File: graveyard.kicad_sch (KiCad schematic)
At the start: 93 parts, among them J30 TX_FILT_IN, J31 To CTRL:ATU, J32 UTF1_OUT, J33 UTF1_IN, J34 UTF1_OUT, J35 UTF1_IN, J36 TX_FILT_OUT, K35 EC2-5SNU, K36 EC2-5SNU, K37 EC2-5SNU, K38 EC2-5SNU, K39 EC2-5SNU, K40 EC2-5SNU, K41 EC2-5SNU, K42 EC2-5SNU, K43 G6E, K44 EC2-5SNU, Q10 BT169B, U17 ULN2803A, U18 MCP23008-xSO, U19 LM555xM

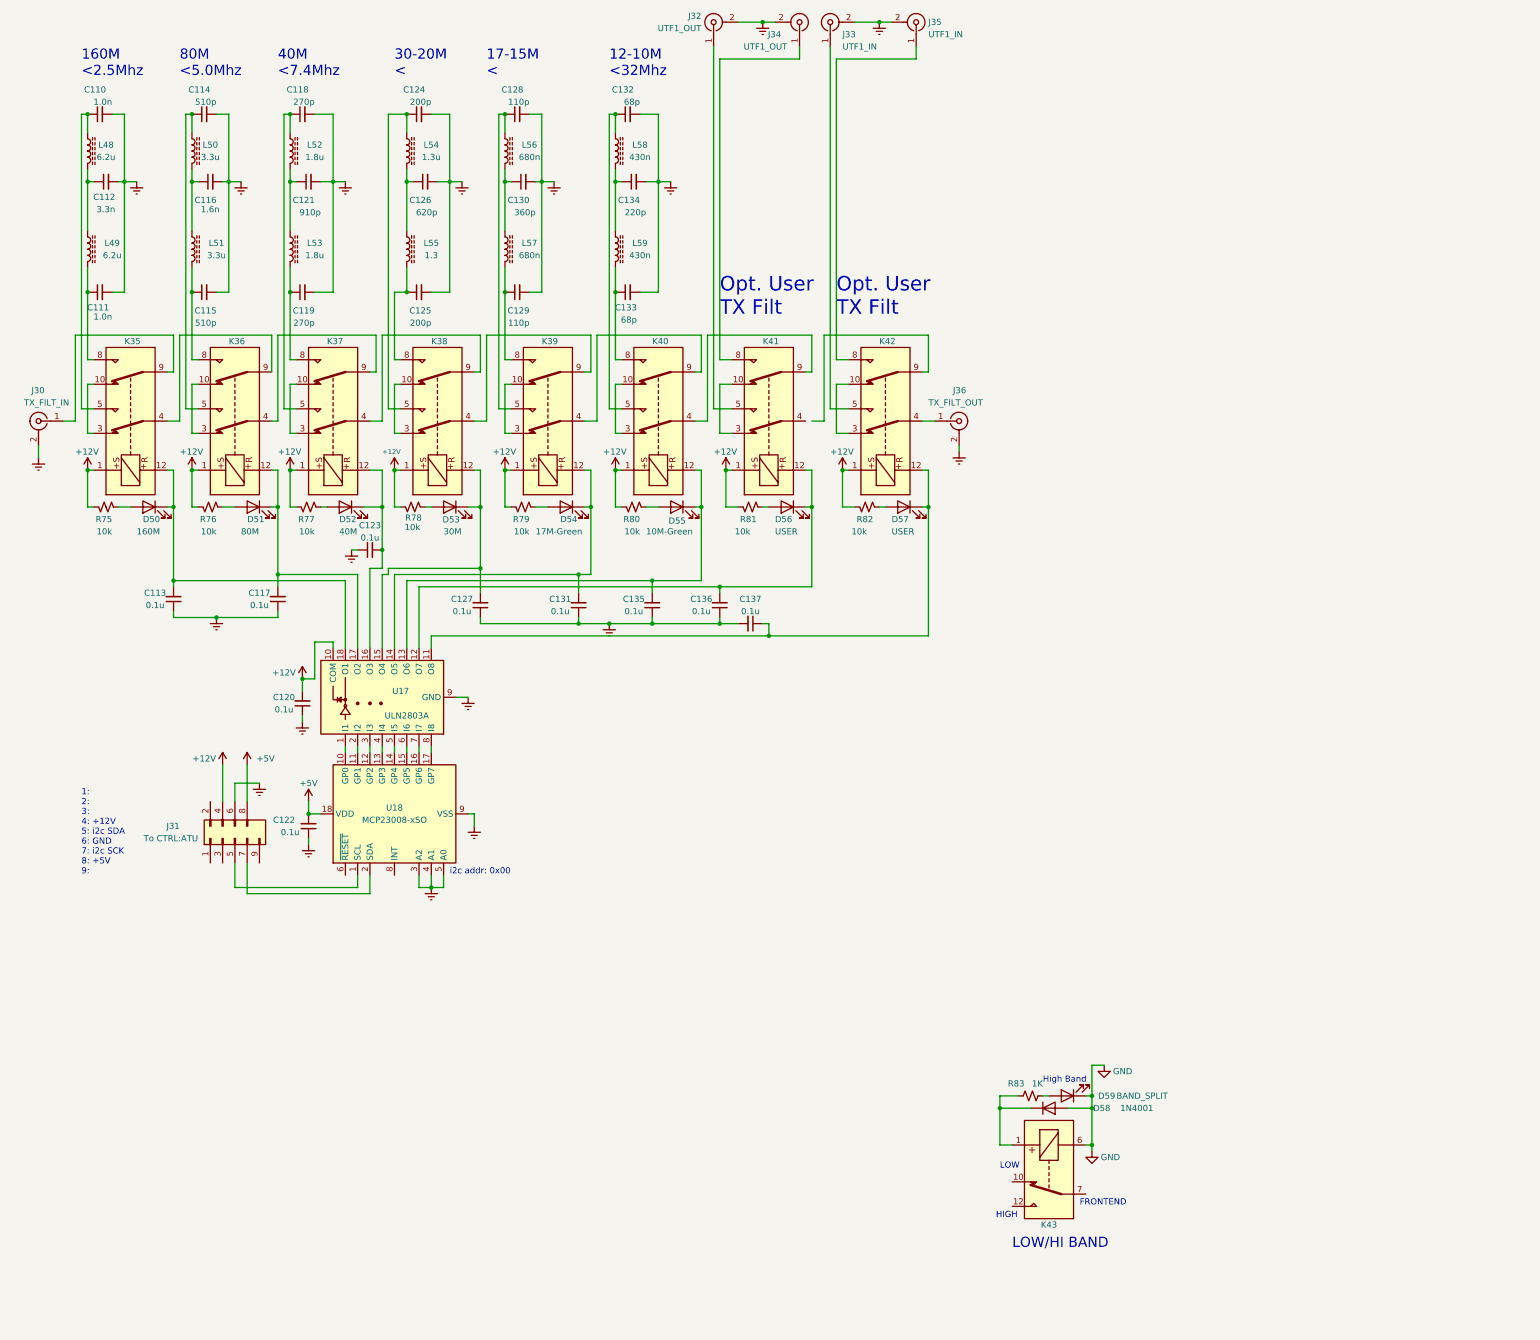
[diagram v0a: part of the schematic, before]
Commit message: cleanup of schematic and some initial firmware works...
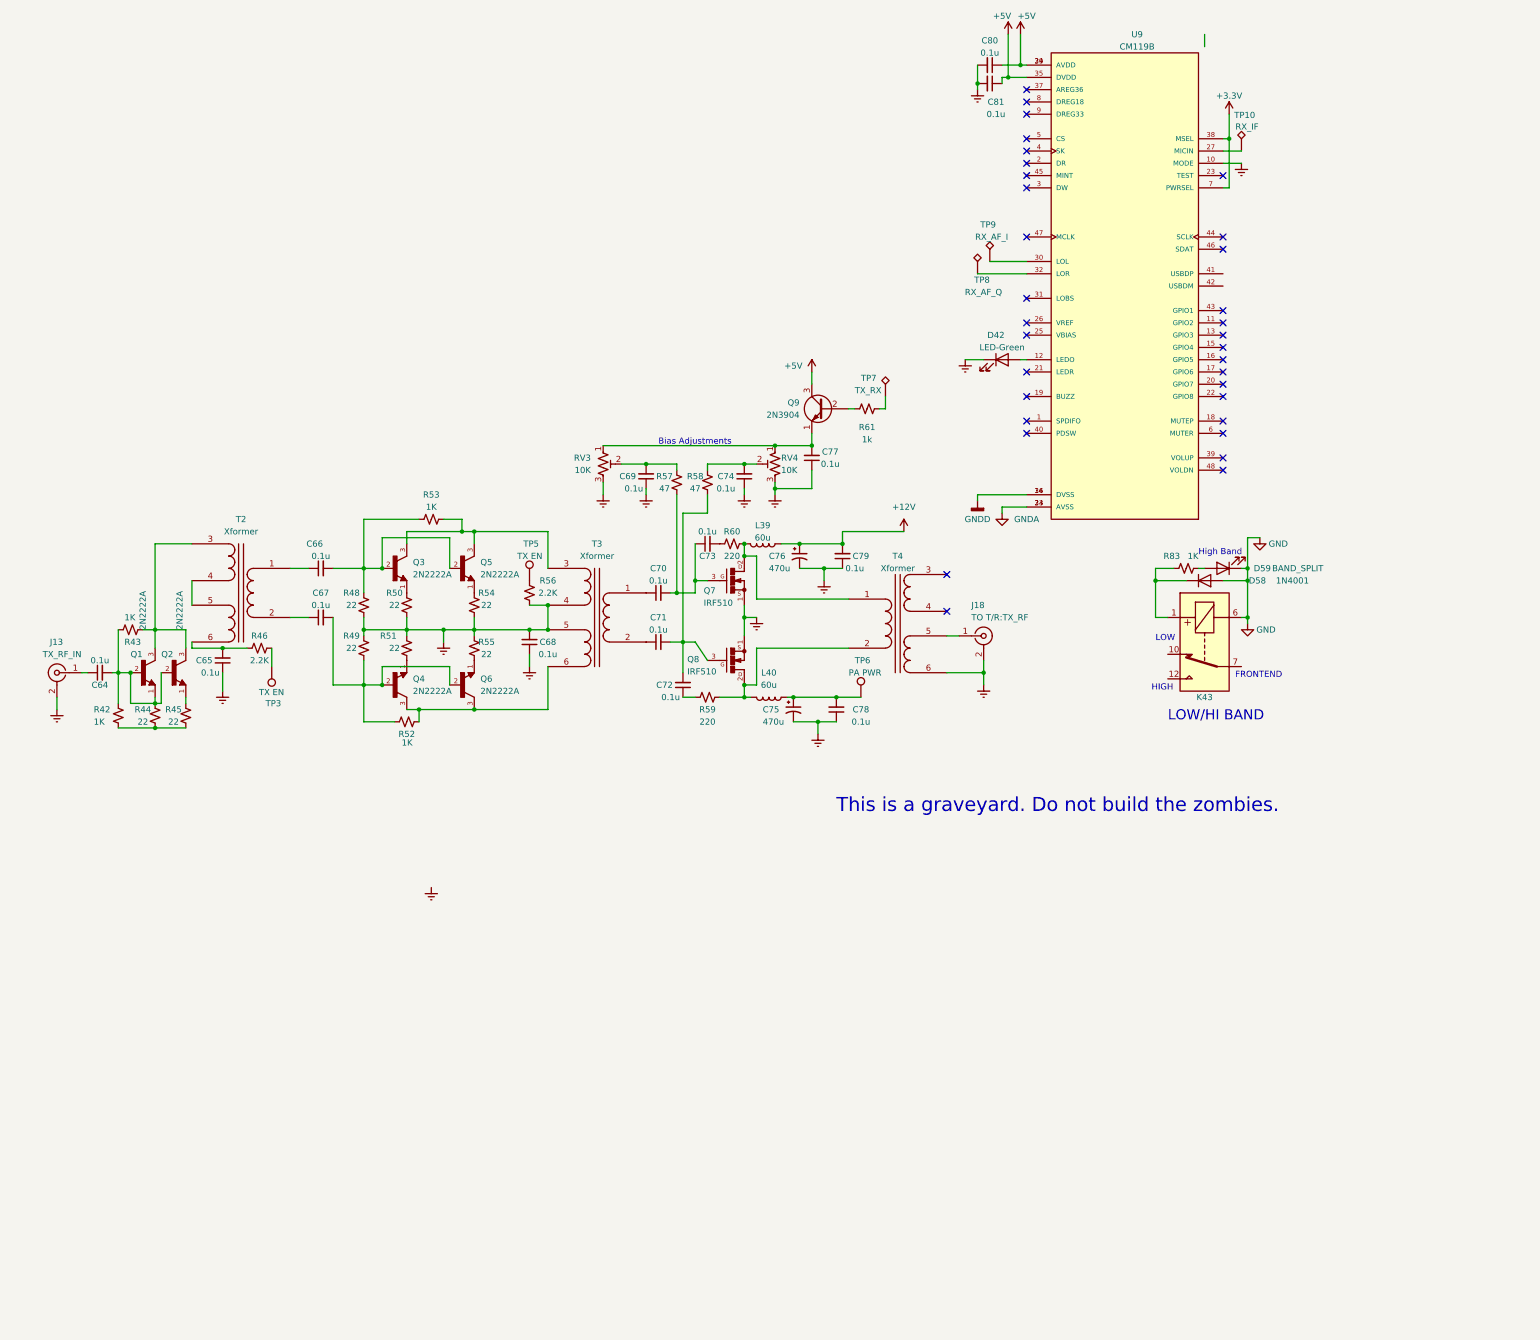
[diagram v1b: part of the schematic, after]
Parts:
- removed C110, C111: 1.0n, symbol Device:C_Small
- removed C112: 3.3n, symbol Device:C_Small
- removed C113, C117, C120, C122, C123, C127, C131, C135, C136, C137: 0.1u, Capacitor_THT:C_Disc_D4.7mm_W2.5mm_P5.00mm, symbol Device:C_Small
- removed C114, C115: 510p, symbol Device:C_Small
- removed C116: 1.6n, symbol Device:C_Small
- removed C118, C119: 270p, symbol Device:C_Small
- removed C121: 910p, symbol Device:C_Small
- removed C124, C125: 200p, symbol Device:C_Small
- removed C126: 620p, symbol Device:C_Small
- removed C128, C129: 110p, symbol Device:C_Small
- removed C130: 360p, symbol Device:C_Small
- removed C132, C133: 68p, symbol Device:C_Small
- removed C134: 220p, symbol Device:C_Small
- removed D50: 160M, symbol Device:LED
- removed D51: 80M, symbol Device:LED
- removed D52: 40M, symbol Device:LED
- removed D53: 30M, symbol Device:LED
- removed D54: 17M-Green, symbol Device:LED
- removed D55: 10M-Green, symbol Device:LED
- removed D56, D57: USER, symbol Device:LED
- removed J30: TX_FILT_IN, symbol Connector:Conn_Coaxial
- removed J31: To CTRL:ATU, symbol Connector_Generic:Conn_2Rows-09Pins
- removed J32, J34: UTF1_OUT, symbol Connector:Conn_Coaxial
- removed J33, J35: UTF1_IN, symbol Connector:Conn_Coaxial
- removed J36: TX_FILT_OUT, symbol Connector:Conn_Coaxial
- removed K35, K36, K37, K38, K39, K40, K41, K42: EC2-5SNU, Relay_THT:Relay_DPDT_Kemet_EC2, symbol Relay:EC2-5SNU
- removed L48, L49: 6.2u, symbol Device:L_Ferrite
- removed L50, L51: 3.3u, symbol Device:L_Ferrite
- removed L52, L53: 1.8u, symbol Device:L_Ferrite
- removed L54: 1.3u, symbol Device:L_Ferrite
- removed L55: 1.3, symbol Device:L_Ferrite
- removed L56, L57: 680n, symbol Device:L_Ferrite
- removed L58, L59: 430n, symbol Device:L_Ferrite
- removed R75, R76, R77, R78, R79, R80, R81, R82: 10k, symbol Device:R_Small_US
- removed U17: ULN2803A, symbol Transistor_Array:ULN2803A
- removed U18: MCP23008-xSO, Package_SO:SOIC-18W_7.5x11.6mm_P1.27mm, symbol Interface_Expansion:MCP23008-xSO
- added C64, C65, C66, C67, C68, C69, C70, C71, C72, C73, C74, C77, C78, C79, C80, C81: 0.1u, Capacitor_THT:C_Disc_D4.7mm_W2.5mm_P5.00mm, symbol Device:C_Small
- added C75, C76: 470u, Capacitor_THT:CP_Radial_D4.0mm_P2.00mm, symbol Device:C_Polarized_Small_US
- added D42: LED-Green, LED_SMD:LED_PLCC_2835_Handsoldering, symbol Device:LED
- added J13: TX_RF_IN, symbol Connector:Conn_Coaxial
- added J18: TO T/R:TX_RF, symbol Connector:Conn_Coaxial
- added L39, L40: 60u, symbol Device:L
- added Q1, Q2, Q3, Q4, Q5, Q6: 2N2222A, TO127P584H533-3, symbol 2N2222A:2N2222A
- added Q7, Q8: IRF510, TO220, symbol IRF510:IRF510
- added Q9: 2N3904, Package_TO_SOT_THT:TO-92_Inline, symbol Transistor_BJT:2N3904
- added R42, R43, R52, R53: 1K, Resistor_THT:R_Axial_DIN0207_L6.3mm_D2.5mm_P2.54mm_Vertical, symbol Device:R_Small_US
- added R44, R45, R48, R49, R50, R51, R54, R55: 22, Resistor_THT:R_Axial_DIN0207_L6.3mm_D2.5mm_P2.54mm_Vertical, symbol Device:R_Small_US
- added R46, R56: 2.2K, Resistor_THT:R_Axial_DIN0207_L6.3mm_D2.5mm_P2.54mm_Vertical, symbol Device:R_Small_US
- added R57, R58: 47, Resistor_THT:R_Axial_DIN0207_L6.3mm_D2.5mm_P2.54mm_Vertical, symbol Device:R_Small_US
- added R59, R60: 220, Resistor_THT:R_Axial_DIN0207_L6.3mm_D2.5mm_P2.54mm_Vertical, symbol Device:R_Small_US
- added R61: 1k, Resistor_THT:R_Axial_DIN0207_L6.3mm_D2.5mm_P2.54mm_Vertical, symbol Device:R_Small_US
- added RV3, RV4: 10K, Potentiometer_THT:Potentiometer_Vishay_T7-YA_Single_Vertical, symbol Device:R_Potentiometer_Trim_US
- added T2, T3, T4: Xformer, symbol Device:Transformer_1P_2S
- added TP10: RX_IF, symbol Connector:TestPoint_Alt
- added TP3, TP5: TX EN, symbol Connector:TestPoint
- added TP6: PA PWR, symbol Connector:TestPoint
- added TP7: TX_RX, symbol Connector:TestPoint_Alt
- added TP8: RX_AF_Q, symbol Connector:TestPoint_Alt
- added TP9: RX_AF_I, symbol Connector:TestPoint_Alt
- added U9: CM119B, Package_QFP:TQFP-48_7x7mm_P0.5mm, symbol CM119B:CM119B
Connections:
- net +12V: now also C76.1, C79.2, L39.1
- net +5V: now also C80.1, C81.1, Q9.3 (C), U9.29 (AVDD), U9.34 (AVDD), U9.35 (DVDD)
- net Earth: now also C65.1, C68.1, C68.2, C69.1, C74.1, C75.2, C76.2, C77.1, C78.1, C79.1, C80.2, C81.2, D42.1 (K), J13.2 (Ext), J18.2 (Ext), Q7.1, Q8.1, R48.1, R49.2, R50.1, R51.2, R54.1, R55.2, R56.1, RV3.3, RV4.3, T3.4 (SB), T3.5 (SC), T4.6 (SD), U9.10 (MODE)
- new net: Q5.1, R54.2
- new net: C66.2, Q3.2, Q5.2, R48.2, R53.1
- new net: Q3.3, Q5.3, R53.2, T3.3 (SA)
- new net: C65.2, R46.1, T2.6 (SD)
- new net: R46.2, TP3.1
- new net: R61.1, TP7.1
- new net: Q9.2 (B), R61.2
- new net: C70.1, T3.1 (AA)
- new net: C71.1, T3.2 (AB)
- new net: Q4.3, Q6.3, R52.2, T3.6 (SD)
- new net: R56.2, TP5.1
- new net: C73.2, R60.1
- new net: L39.2, Q7.2, R60.2, T4.1 (AA)
- new net: C70.2, C73.1, Q7.3, R57.1
- new net: C66.1, T2.1 (AA)
- new net: C67.1, T2.2 (AB)
- new net: Q1.3, Q2.3, R43.1, T2.3 (SA)
- new net: T2.4 (SB), T2.5 (SC)
- new net: Q3.1, R50.2
- new net: R42.2, R44.1, R45.1
- new net: C64.2, Q1.1, Q1.2, Q2.2, R42.1, R43.2, R44.2
- new net: C69.2, R57.2, RV3.2
- new net: C67.2, Q4.2, Q6.2, R49.1, R52.1
- new net: Q2.1, R45.2
- new net: J18.1 (In), T4.5 (SC)
- new net: C77.2, Q9.1 (E), RV3.1, RV4.1
- new net: C71.2, C72.2, Q8.3, R58.1
- new net: TP8.1, U9.32 (LOR)
- new net: L40.2, Q8.2, R59.2, T4.2 (AB)
- new net: C64.1, J13.1 (In)
- new net: C75.1, C78.2, L40.1, TP6.1
- new net: C74.2, R58.2, RV4.2
- new net: TP10.1, U9.27 (MICIN)
- new net: D42.2 (A), U9.12 (LEDO)
- new net: TP9.1, U9.30 (LOL)
- new net: C72.1, R59.1
- new net: Q6.1, R55.1
- new net: Q4.1, R51.1
- new net +3.3V: U9.38 (MSEL), U9.7 (PWRSEL)
- new net GNDA: U9.24 (AVSS), U9.33 (AVSS)
- new net GNDD: U9.14 (DVSS), U9.36 (DVSS)
- no-connect marks 0 -> 33
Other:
- note added: "Bias Adjustments"
- note added: "This is a graveyard. Do not build the zombies."
- note removed: "12-10M <32Mhz"
- note removed: "160M <2.5Mhz"
- note removed: "17-15M <"
- note removed: "1: 2: 3: 4: +12V 5: i2c SDA 6: GND 7: i2c SCK 8: +5V 9:"
- note removed: "30-20M <"
- note removed: "40M <7.4Mhz"
- note removed: "80M <5.0Mhz"
- note removed: "Opt. User TX Filt"
- note removed: "i2c addr: 0x00"
- moved on the sheet: D58, D59, K43, R83
